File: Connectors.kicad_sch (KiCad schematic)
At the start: 13 parts, among them J5 Conn_02x03_Odd_Even, J6 Conn_02x03_Odd_Even, U12 TJA1051T/3

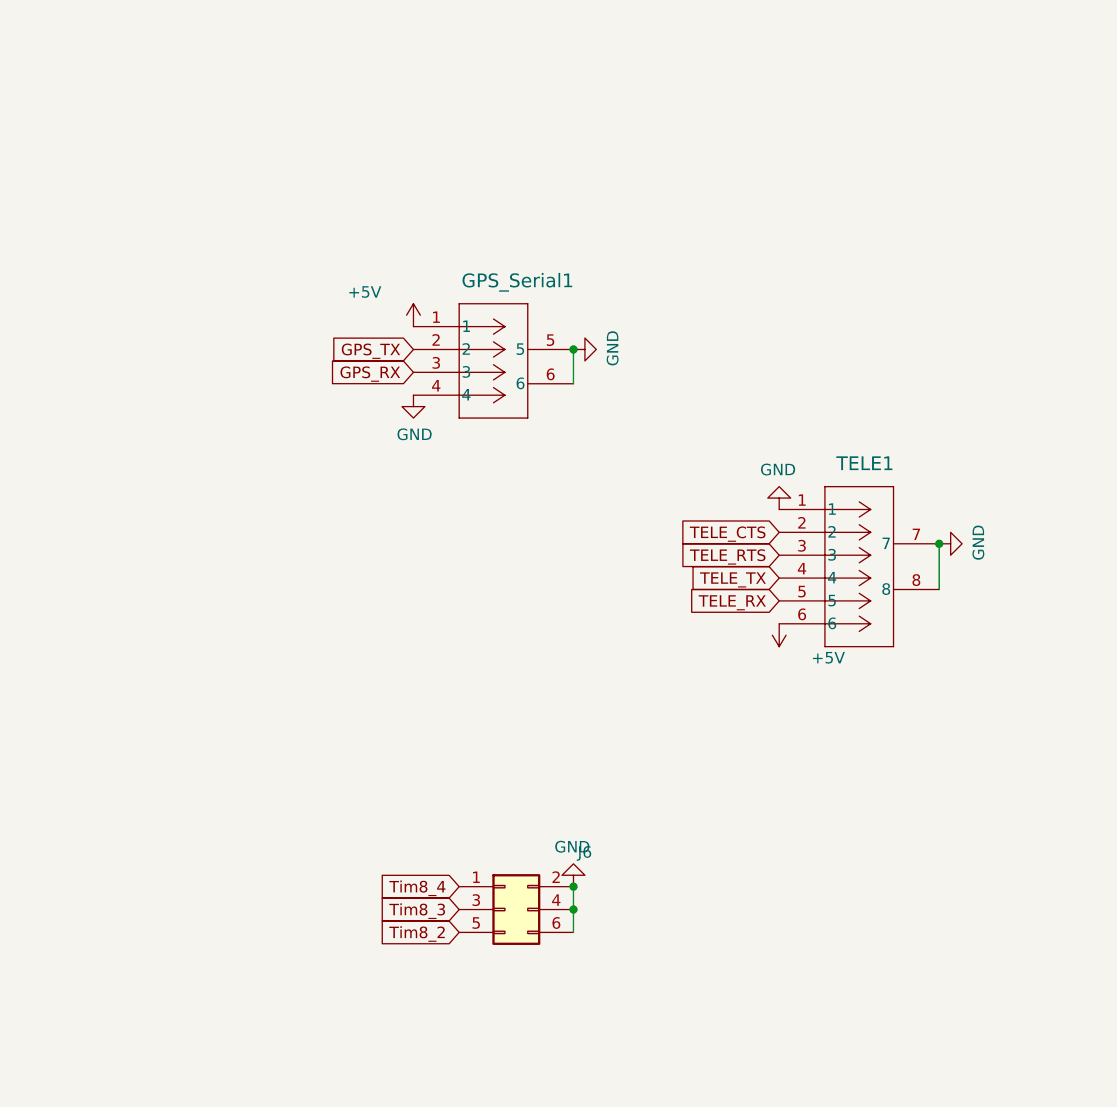
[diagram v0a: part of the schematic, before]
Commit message: update
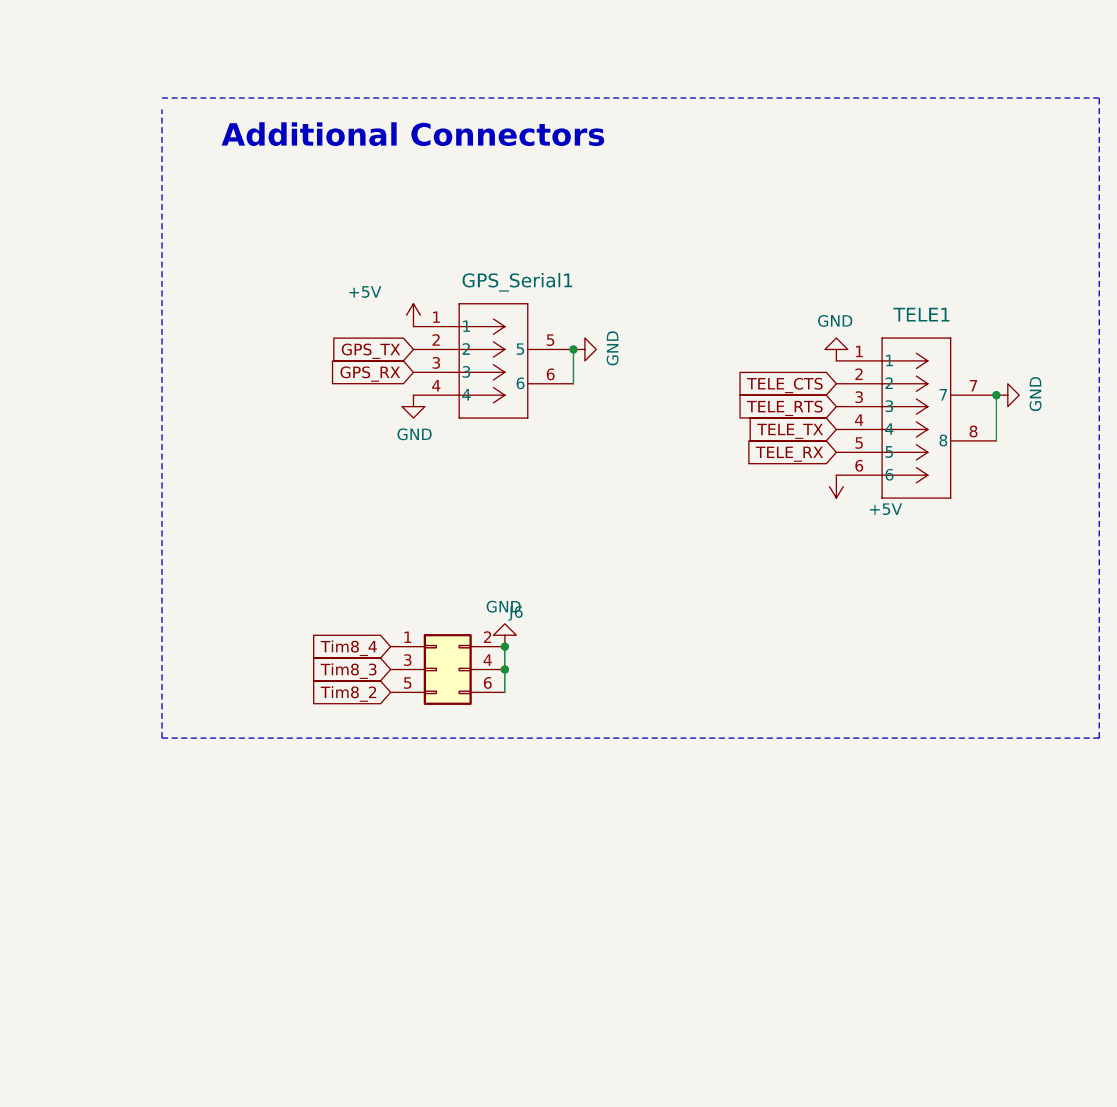
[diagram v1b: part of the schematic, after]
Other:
- note added: "Additional Connectors"
- moved on the sheet: J6, TELE1
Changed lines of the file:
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@@
 	(generator_version "9.0")
 	(paper "A4")
+	(text "Additional Connectors\n"
+		(exclude_from_sim no)
+		(at 180.594 38.862 0)
+		(effects
+			(font
+				(size 2.4892 2.4892)
+				(thickness 0.4978)
+				(bold yes)
+			)
+			(justify left bottom)
+		)
+	)
 	(text "SWD"
 		(exclude_from_sim no)
@@
 	)
 	(junction
-		(at 260.35 82.55)
+		(at 266.7 66.04)
 		(diameter 0)
 		(color 0 0 0 0)
@@
 	)
 	(junction
-		(at 219.71 120.65)
+		(at 212.09 93.98)
 		(diameter 0)
 		(color 0 0 0 0)
@@
 	)
 	(junction
-		(at 219.71 123.19)
+		(at 212.09 96.52)
 		(diameter 0)
 		(color 0 0 0 0)
@@
 	(wire
 		(pts
-			(xy 260.35 82.55) (xy 260.35 87.63)
+			(xy 266.7 66.04) (xy 266.7 71.12)
 		)
 		(stroke
@@
 		)
 	)
+	(polyline
+		(pts
+			(xy 173.99 33.02) (xy 278.13 33.02)
+		)
+		(stroke
+			(width 0)
+			(type dash)
+		)
+	)
 	(wire
 		(pts
@@
 		)
 	)
+	(polyline
+		(pts
+			(xy 278.13 104.14) (xy 173.99 104.14)
+		)
+		(stroke
+			(width 0)
+			(type dash)
+		)
+	)
 	(wire
 		(pts
@@
 		)
 	)
+	(polyline
+		(pts
+			(xy 278.13 104.14) (xy 278.13 33.02)
+		)
+		(stroke
+			(width 0)
+			(type dash)
+		)
+	)
 	(wire
 		(pts
@@
 	(wire
 		(pts
-			(xy 219.71 123.19) (xy 219.71 125.73)
+			(xy 212.09 96.52) (xy 212.09 99.06)
 		)
 		(stroke
@@
 		)
 	)
+	(polyline
+		(pts
+			(xy 173.99 104.14) (xy 173.99 34.2899)
+		)
+		(stroke
+			(width 0)
+			(type dash)
+		)
+	)
 	(wire
 		(pts
@@
 	(wire
 		(pts
-			(xy 219.71 120.65) (xy 219.71 123.19)
+			(xy 212.09 93.98) (xy 212.09 96.52)
 		)
 		(stroke
@@
 	(global_label "Tim8_4"
 		(shape input)
-		(at 207.01 120.65 180)
+		(at 199.39 93.98 180)
 		(effects
 			(font
@@
 		)
 		(property "Intersheetrefs" "${INTERSHEET_REFS}"
-			(at 207.01 120.65 0)
+			(at 199.39 93.98 0)
 			(effects
 				(font
@@
 	(global_label "TELE_CTS"
 		(shape input)
-		(at 242.57 81.28 180)
+		(at 248.92 64.77 180)
 		(effects
 			(font
@@
 		)
 		(property "Intersheetrefs" "${INTERSHEET_REFS}"
-			(at 242.57 81.28 0)
+			(at 248.92 64.77 0)
 			(effects
 				(font
@@
 	(global_label "TELE_RX"
 		(shape input)
-		(at 242.57 88.9 180)
+		(at 248.92 72.39 180)
 		(effects
 			(font
@@
 		)
 		(property "Intersheetrefs" "${INTERSHEET_REFS}"
-			(at 242.57 88.9 0)
+			(at 248.92 72.39 0)
 			(effects
 				(font
@@
 	(global_label "TELE_TX"
 		(shape input)
-		(at 242.57 86.36 180)
+		(at 248.92 69.85 180)
 		(effects
 			(font
@@
 		)
 		(property "Intersheetrefs" "${INTERSHEET_REFS}"
-			(at 242.57 86.36 0)
+			(at 248.92 69.85 0)
 			(effects
 				(font
@@
 	(global_label "TELE_RTS"
 		(shape input)
-		(at 242.57 83.82 180)
+		(at 248.92 67.31 180)
 		(effects
 			(font
@@
 		)
 		(property "Intersheetrefs" "${INTERSHEET_REFS}"
-			(at 242.57 83.82 0)
+			(at 248.92 67.31 0)
 			(effects
 				(font
@@
 	(global_label "Tim8_2"
 		(shape input)
-		(at 207.01 125.73 180)
+		(at 199.39 99.06 180)
 		(effects
 			(font
@@
 		)
 		(property "Intersheetrefs" "${INTERSHEET_REFS}"
-			(at 207.01 125.73 0)
+			(at 199.39 99.06 0)
 			(effects
 				(font
@@
 	(global_label "Tim8_3"
 		(shape input)
-		(at 207.01 123.19 180)
+		(at 199.39 96.52 180)
 		(effects
 			(font
@@
 		)
 		(property "Intersheetrefs" "${INTERSHEET_REFS}"
-			(at 207.01 123.19 0)
+			(at 199.39 96.52 0)
 			(effects
 				(font
@@
 	(symbol
 		(lib_id "power:GND")
-		(at 242.57 78.74 180)
+		(at 248.92 62.23 180)
 		(unit 1)
 		(exclude_from_sim no)
@@
 		(dnp no)
 		(property "Reference" "#PWR096"
-			(at 242.57 72.39 0)
+			(at 248.92 55.88 0)
 			(effects
 				(font
@@
 		)
 		(property "Value" "GND"
-			(at 242.443 74.3458 0)
+			(at 248.793 57.8358 0)
 			(effects
 				(font
@@
 		)
 		(property "Footprint" ""
-			(at 242.57 78.74 0)
+			(at 248.92 62.23 0)
 			(effects
 				(font
@@
 		)
 		(property "Datasheet" ""
-			(at 242.57 78.74 0)
+			(at 248.92 62.23 0)
 			(effects
 				(font
@@
 		)
 		(property "Description" "Power symbol creates a global label with name \"GND\" , ground"
-			(at 242.57 78.74 0)
+			(at 248.92 62.23 0)
 			(effects
 				(font
@@
 	(symbol
 		(lib_id "power:+5V")
-		(at 242.57 91.44 180)
+		(at 248.92 74.93 180)
 		(unit 1)
 		(exclude_from_sim no)
@@
 		(dnp no)
 		(property "Reference" "#PWR097"
-			(at 242.57 87.63 0)
+			(at 248.92 71.12 0)
 			(effects
 				(font
@@
 		)
 		(property "Value" "+5V"
-			(at 246.126 95.25 0)
+			(at 252.476 78.74 0)
 			(effects
 				(font
@@
 		)
 		(property "Footprint" ""
-			(at 242.57 91.44 0)
+			(at 248.92 74.93 0)
 			(effects
 				(font
@@
 		)
 		(property "Datasheet" ""
-			(at 242.57 91.44 0)
+			(at 248.92 74.93 0)
 			(effects
 				(font
@@
 		)
 		(property "Description" "Power symbol creates a global label with name \"+5V\""
-			(at 242.57 91.44 0)
+			(at 248.92 74.93 0)
 			(effects
 				(font
@@
 	(symbol
 		(lib_id "power:GND")
-		(at 260.35 82.55 90)
+		(at 266.7 66.04 90)
 		(unit 1)
 		(exclude_from_sim no)
@@
 		(dnp no)
 		(property "Reference" "#PWR098"
-			(at 266.7 82.55 0)
+			(at 273.05 66.04 0)
 			(effects
 				(font
@@
 		)
 		(property "Value" "GND"
-			(at 264.7442 82.423 0)
+			(at 271.0942 65.913 0)
 			(effects
 				(font
@@
 		)
 		(property "Footprint" ""
-			(at 260.35 82.55 0)
+			(at 266.7 66.04 0)
 			(effects
 				(font
@@
 		)
 		(property "Datasheet" ""
-			(at 260.35 82.55 0)
+			(at 266.7 66.04 0)
 			(effects
 				(font
@@
 		)
 		(property "Description" "Power symbol creates a global label with name \"GND\" , ground"
-			(at 260.35 82.55 0)
+			(at 266.7 66.04 0)
 			(effects
 				(font
@@
 	(symbol
 		(lib_id "SM06B-GHS-TB:SM06B-GHS-TB")
-		(at 242.57 78.74 0)
+		(at 248.92 62.23 0)
 		(unit 1)
 		(exclude_from_sim no)
@@
 		(dnp no)
 		(property "Reference" "TELE1"
-			(at 248.92 73.66 0)
+			(at 255.27 57.15 0)
 			(effects
 				(font
@@
 		)
 		(property "Value" "SM06B-GHS-TB"
-			(at 256.54 86.3599 0)
+			(at 262.89 69.8499 0)
 			(effects
 				(font
@@
 		)
 		(property "Footprint" "mylib:CONN_SM06B-GHS-TB_JST"
-			(at 242.57 78.74 0)
+			(at 248.92 62.23 0)
 			(effects
 				(font
@@
 		)
 		(property "Datasheet" "SM06B-GHS-TB"
-			(at 242.57 78.74 0)
+			(at 248.92 62.23 0)
 			(effects
 				(font
@@
 		)
 		(property "Description" ""
-			(at 242.57 78.74 0)
+			(at 248.92 62.23 0)
 			(effects
 				(font
@@
 	(symbol
 		(lib_id "power:GND")
-		(at 219.71 120.65 180)
+		(at 212.09 93.98 180)
 		(unit 1)
 		(exclude_from_sim no)
@@
 		(dnp no)
 		(property "Reference" "#PWR095"
-			(at 219.71 114.3 0)
+			(at 212.09 87.63 0)
 			(effects
 				(font
@@
 		)
 		(property "Value" "GND"
-			(at 219.583 116.2558 0)
+			(at 211.963 89.5858 0)
 			(effects
 				(font
@@
 		)
 		(property "Footprint" ""
-			(at 219.71 120.65 0)
+			(at 212.09 93.98 0)
 			(effects
 				(font
@@
 		)
 		(property "Datasheet" ""
-			(at 219.71 120.65 0)
+			(at 212.09 93.98 0)
 			(effects
 				(font
@@
 		)
 		(property "Description" "Power symbol creates a global label with name \"GND\" , ground"
-			(at 219.71 120.65 0)
+			(at 212.09 93.98 0)
 			(effects
 				(font
@@
 	(symbol
 		(lib_id "Connector_Generic:Conn_02x03_Odd_Even")
-		(at 212.09 123.19 0)
+		(at 204.47 96.52 0)
 		(unit 1)
 		(exclude_from_sim no)
@@
 		(dnp no)
 		(property "Reference" "J6"
-			(at 220.98 116.84 0)
+			(at 213.36 90.17 0)
 			(effects
 				(font
@@
 		)
 		(property "Value" "Conn_02x03_Odd_Even"
-			(at 213.36 116.84 0)
+			(at 205.74 90.17 0)
 			(effects
 				(font
@@
 		)
 		(property "Footprint" "Connector_PinSocket_2.00mm:PinSocket_2x03_P2.00mm_Vertical"
-			(at 212.09 123.19 0)
+			(at 204.47 96.52 0)
 			(effects
 				(font
@@
 		)
 		(property "Datasheet" "~"
-			(at 212.09 123.19 0)
+			(at 204.47 96.52 0)
 			(effects
 				(font
@@
 		)
 		(property "Description" "Generic connector, double row, 02x03, odd/even pin numbering scheme (row 1 odd numbers, row 2 even numbers), script generated (kicad-library-utils/schlib/autogen/connector/)"
-			(at 212.09 123.19 0)
-			(effects
-				(font
+			(at 204.47 96.52 0)
+			(effects
+				(font

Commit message: update
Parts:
- R19: LCSC Part (none) -> C166918
- R20: LCSC (none) -> C166918
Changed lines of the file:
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@@
 			)
 		)
-		(property "Description" "Resistor"
+		(property "Description" "Resistor RALEC RTT0360R0FTP"
+			(at 85.09 74.93 0)
+			(effects
+				(font
+					(size 1.27 1.27)
+				)
+				(hide yes)
+			)
+		)
+		(property "LCSC Part" "C166918"
 			(at 85.09 74.93 0)
 			(effects
@@
 			)
 		)
-		(property "Description" "Resistor"
+		(property "Description" "Resistor RTT0360R0FTP"
 			(at 95.25 74.93 0)
 			(effects
+				(font
+					(size 1.27 1.27)
+				)
+				(hide yes)
+			)
+		)
+		(property "LCSC" "C166918"
+			(at 95.25 74.93 0)
+			(effects

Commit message: PumbaaV2_RC2
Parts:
- CAN1, GPS_Serial1: value SM04B-GHS-TB -> SM04B-GHS-TB(LF)(SN)
- TELE1: value SM06B-GHS-TB -> SM06B-GHS-TB(LF)(SN)
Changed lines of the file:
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@@
 			)
 		)
-		(property "Value" "SM04B-GHS-TB"
+		(property "Value" "SM04B-GHS-TB(LF)(SN)"
 			(at 215.9 63.4999 0)
 			(effects
@@
 			)
 		)
-		(property "Value" "SM06B-GHS-TB"
+		(property "Value" "SM06B-GHS-TB(LF)(SN)"
 			(at 262.89 69.8499 0)
 			(effects
@@
 			)
 		)
-		(property "Value" "SM04B-GHS-TB"
+		(property "Value" "SM04B-GHS-TB(LF)(SN)"
 			(at 123.19 68.5799 0)
 			(effects
